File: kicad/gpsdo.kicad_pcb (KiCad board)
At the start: 2 copper layers, 76.2 x 30.5 mm, 45 parts, among them J1 Conn_Coaxial, J2 Conn_01x04_Male, J3 Conn_01x04_Male, J4 Conn_01x04_Male, J5 Conn_01x04_Male, J6 Conn_01x04_Male, U1 MSP430F5171IDA, U10 74AUC1G79, U11 47L64, U2 MAX-8Q, U3 549CAAC000111BBG, U4 Si7051-A20, U6 74LVC1G08, U7 74LVC1G08, U8 74AUC1G79, U9 74LVC1G86

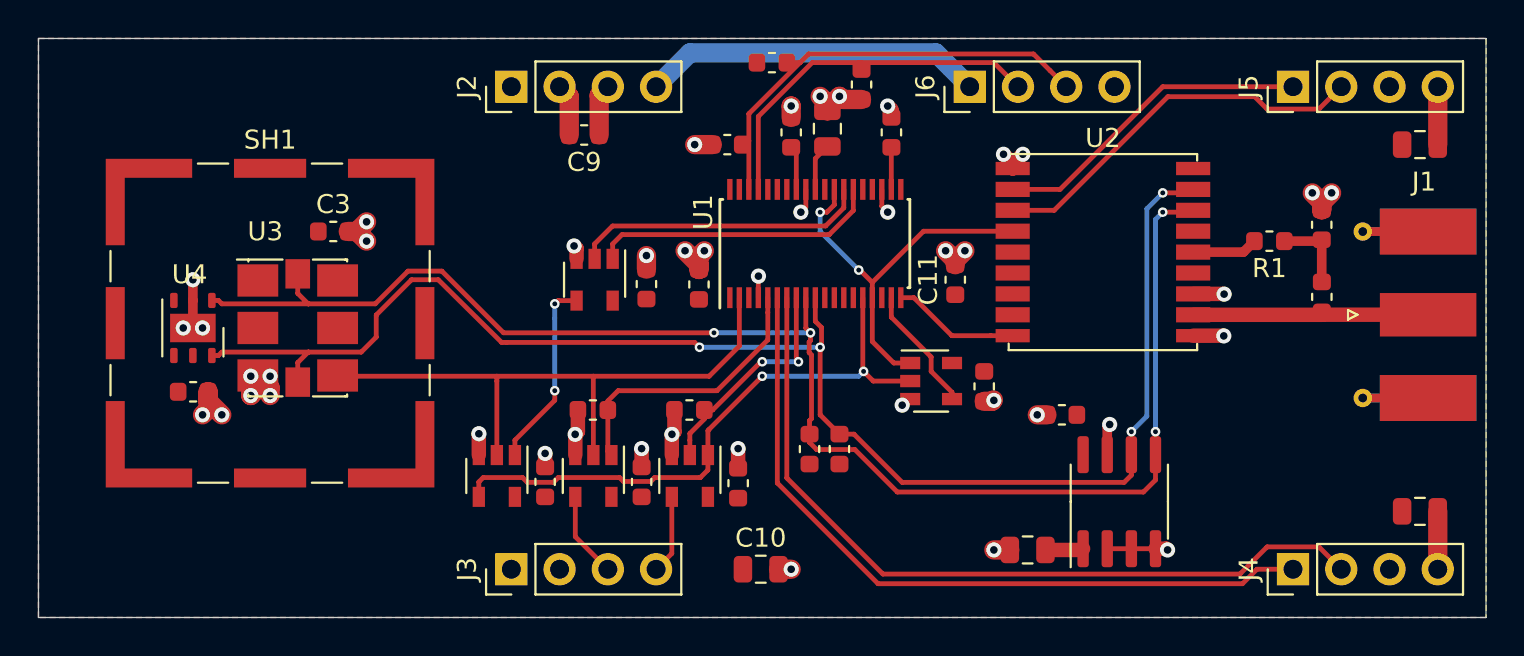
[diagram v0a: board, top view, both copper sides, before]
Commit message: update pcb layout
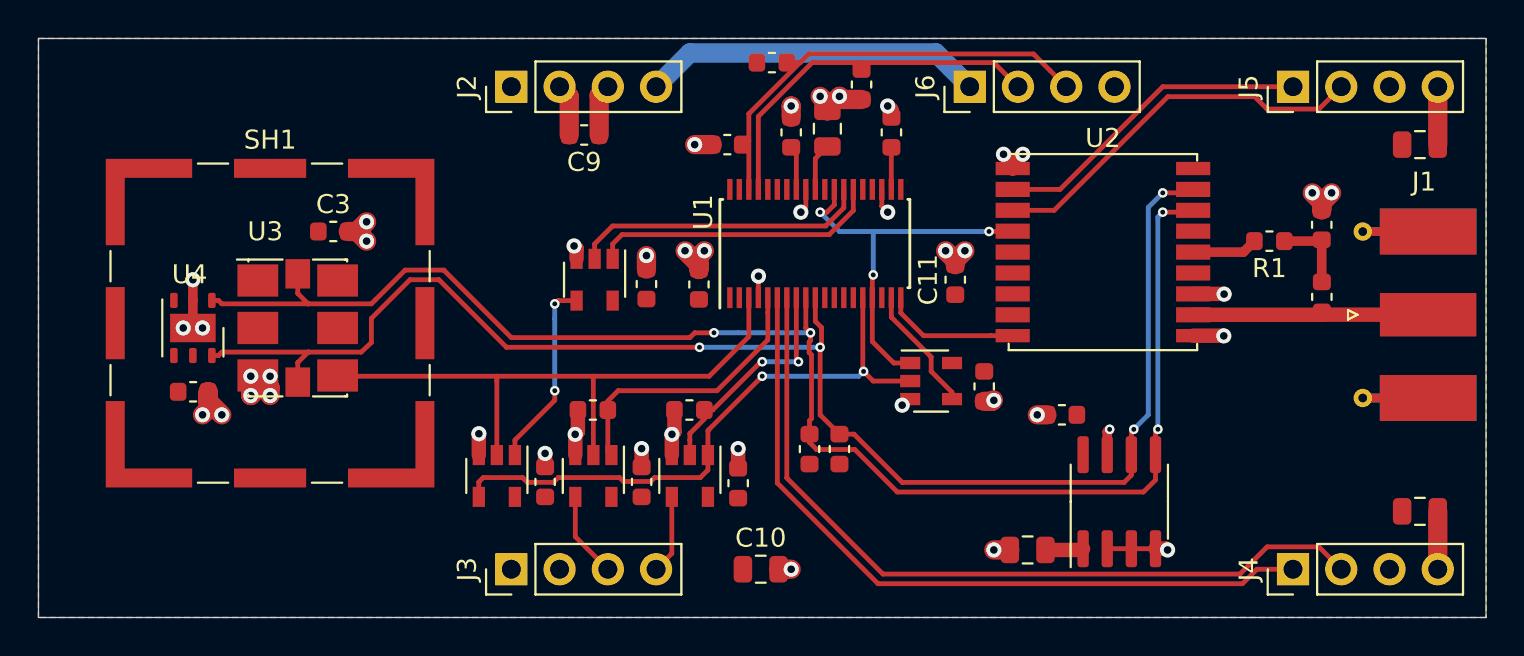
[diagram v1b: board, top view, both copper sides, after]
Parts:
- C10, C19, C20: value 10u -> 22u
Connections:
- net Net-(J1-Pad1) renamed /gANT
- net Net-(U1-Pad19) renamed /gRST
- net Net-(U8-Pad1) renamed /uPPS
- U1 pad 11: Net-(U1-Pad11) -> +3V3
- U1 pad 12: Net-(U1-Pad12) -> +3V3
- U1 pad 13: Net-(U1-Pad13) -> +3V3
- U1 pad 14: Net-(U1-Pad14) -> +3V3
- U1 pad 2: CLK_25M -> Net-(U1-Pad2)
- U1 pad 20: Net-(U1-Pad20) -> +3V3
- U1 pad 23: Net-(U1-Pad23) -> +3V3
- U1 pad 24: Net-(U1-Pad24) -> +3V3
- U1 pad 3: Net-(U1-Pad3) -> CLK_25M
- U1 pad 32: Net-(U1-Pad32) -> +3V3
- U1 pad 33: Net-(U1-Pad33) -> +3V3
- U1 pad 34: Net-(U1-Pad34) -> +3V3
- U1 pad 37: Net-(U1-Pad37) -> +3V3
- U1 pad 38: Net-(U1-Pad38) -> +3V3
- U11 pad 7: Net-(U11-Pad7) -> GND
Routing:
- net Net-(U11-Pad7): track 1.64 -> 0.00 mm, vias 1 -> 0
- net GND: track 56.1 -> 57.5 mm, vias 43 -> 44
- net gPPS: track 20.7 -> 20.6 mm, vias 2 -> 3
